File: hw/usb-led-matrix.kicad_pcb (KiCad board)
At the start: 4 copper layers, 48 x 30 mm, 101 parts, among them J1 USB4085-GF-A, J2 Conn_ST_STDC14, U1 AP2210K-3.3, U2 STM32G473CET6, U3 74LVT245, U4 USBLC6-2SC6, Y1 ABM8-24.000MHZ-B2-T

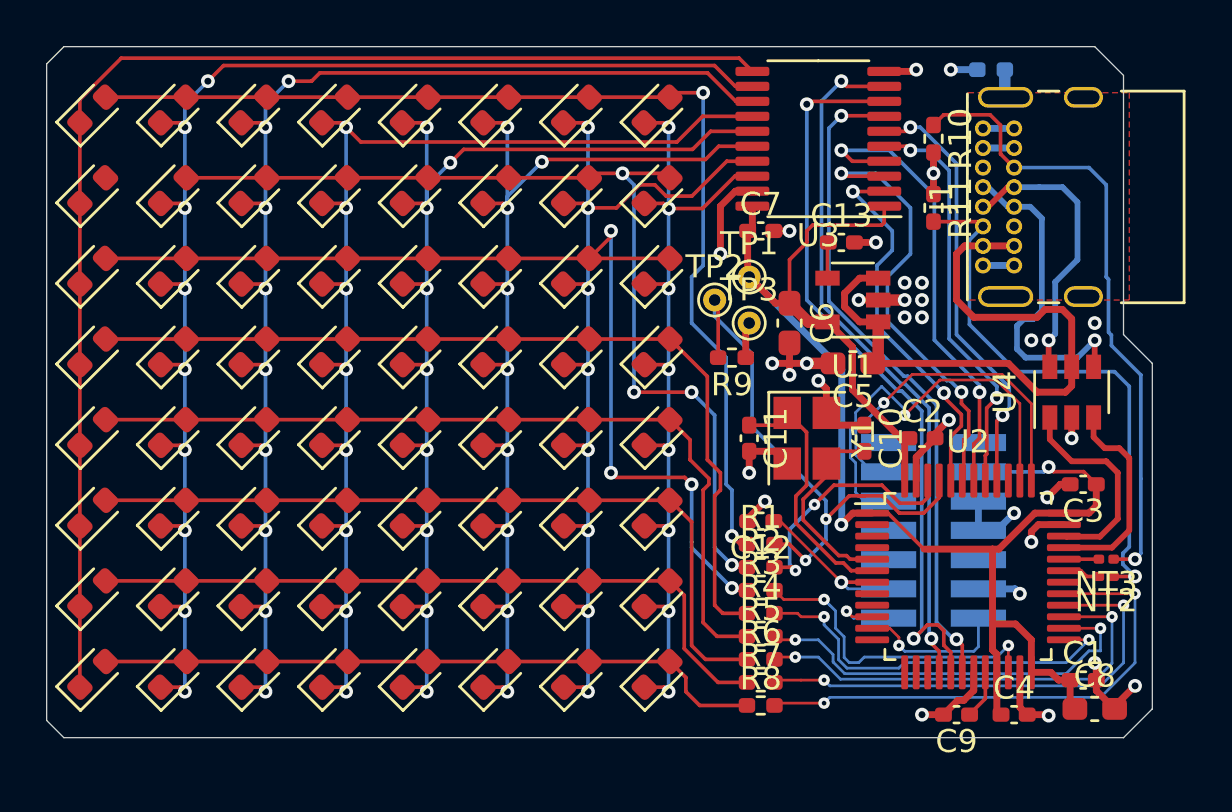
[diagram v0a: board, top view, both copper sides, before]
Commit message: Update routing
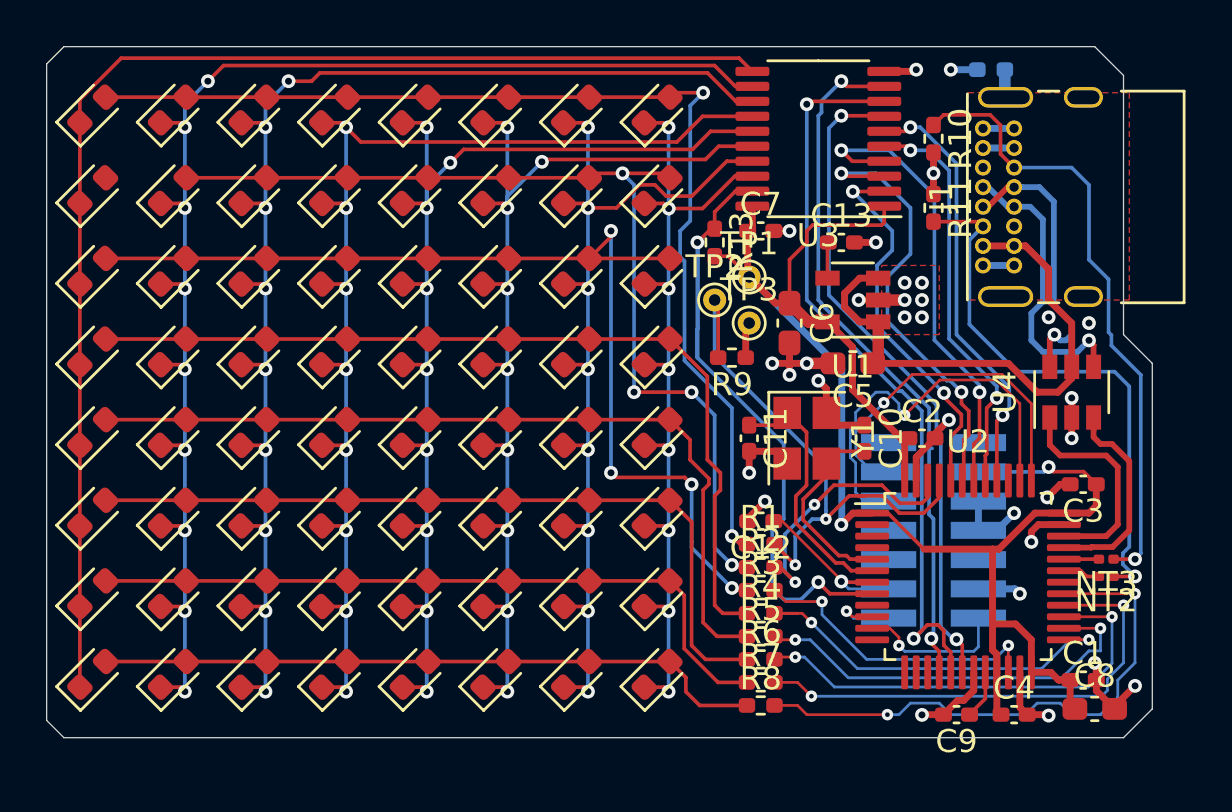
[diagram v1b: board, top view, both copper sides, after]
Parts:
- added R13: R, Resistor_SMD:R_0402_1005Metric_Pad0.72x0.64mm_HandSolder, F.Cu at (169.0, 88.5)
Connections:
- net /USB_DM renamed /USB_D-
- net /USB_DM_CON renamed /USBCON_D-
- net /USB_DP renamed /USB_D+
- net /USB_DP_CON renamed /USBCON_D+
- U2 pad 8: (no net) -> /BUFFER_EN
- U3 pad 19: GND -> /BUFFER_EN
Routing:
- net /BUFFER_EN: track 0.00 -> 30.6 mm, vias 0 -> 2
- net /VBUS: track 29.7 -> 25.1 mm
- net GND: track 49.6 -> 46.7 mm
- net /VDD: track 69.3 -> 71.2 mm
- net /ROW8: track 22.5 -> 24.2 mm
- net /USBCON_D-: track 14.5 -> 12.9 mm
- net /ROW2: track 10.8 -> 11.7 mm
- net /ROW3: track 13.9 -> 13.1 mm
- net /ROW7: track 20.8 -> 21.5 mm
- added copper zone on F.Cu, net GND
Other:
- net class USB: clearance 0.15 -> 0.2
